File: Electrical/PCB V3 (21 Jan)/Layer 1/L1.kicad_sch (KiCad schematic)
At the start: 218 parts, among them J1 Conn_01x05, Q1 NMOS, U1 LM2587S-ADJ, U2 CD74HC4067SM, U3 CD74HC4067SM, U4 XT30UPB-M, U5 113991054

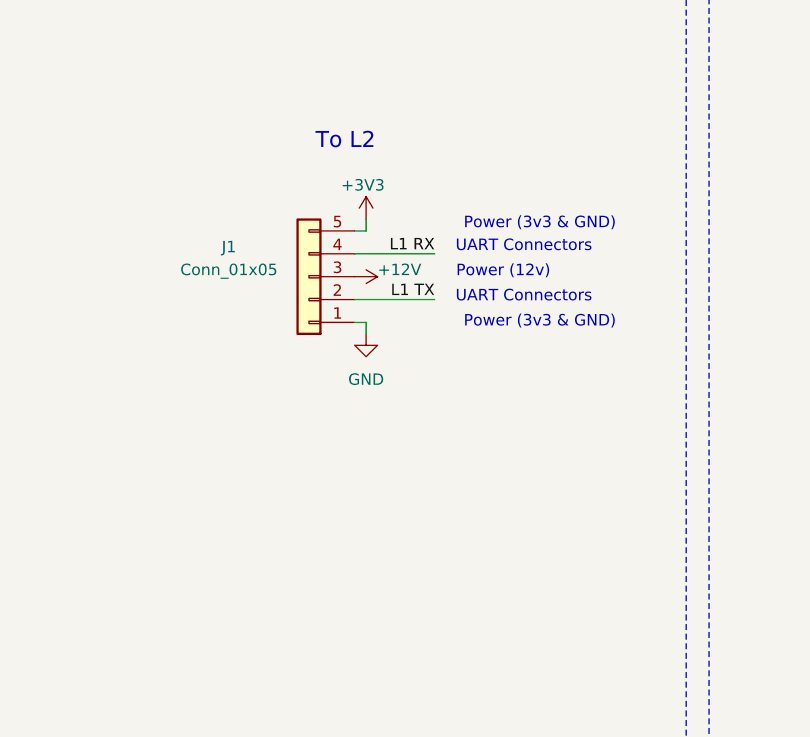
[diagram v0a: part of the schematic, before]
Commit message: 2 new jsts
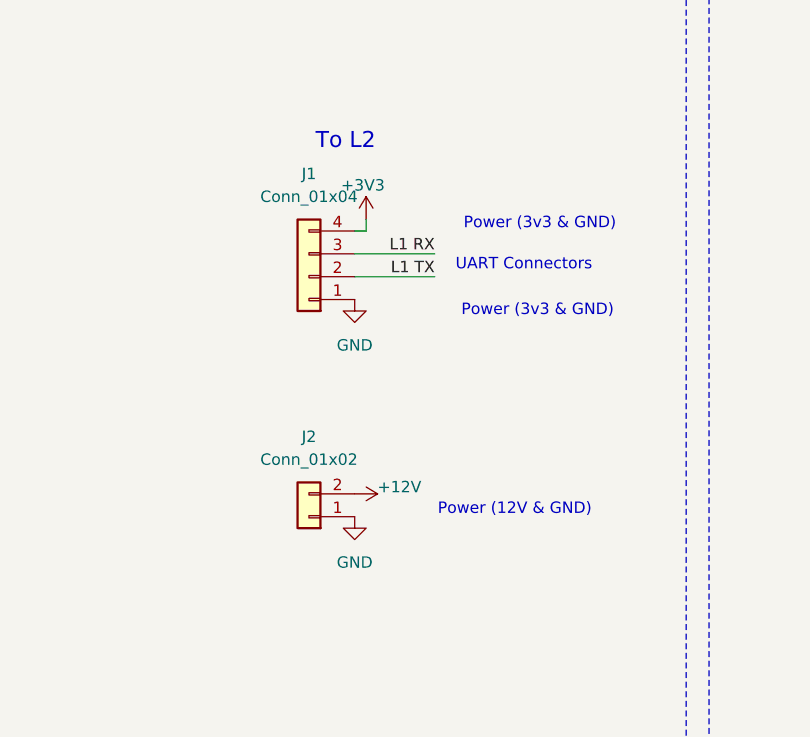
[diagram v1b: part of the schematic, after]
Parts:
- removed J1: Conn_01x05, Connector_JST:JST_EH_B5B-EH-A_1x05_P2.50mm_Vertical, symbol Connector_Generic:Conn_01x05
- added J1: Conn_01x04, Connector_JST:JST_EH_B4B-EH-A_1x04_P2.50mm_Vertical, symbol Connector_Generic:Conn_01x04
- added J2: Conn_01x02, Connector_JST:JST_EH_B2B-EH-A_1x02_P2.50mm_Vertical, symbol Connector_Generic:Conn_01x02
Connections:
- net +12V: now also J2.2 (Pin_2)
- net +3V3: now also J1.4 (Pin_4)
- net GND: now also J1.1 (Pin_1), J2.1 (Pin_1)
- net L1 RX: now also J1.3 (Pin_3)
- net L1 TX: now also J1.2 (Pin_2)
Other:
- note added: "Power (12V & GND)"
- note removed: "Power (12v)"

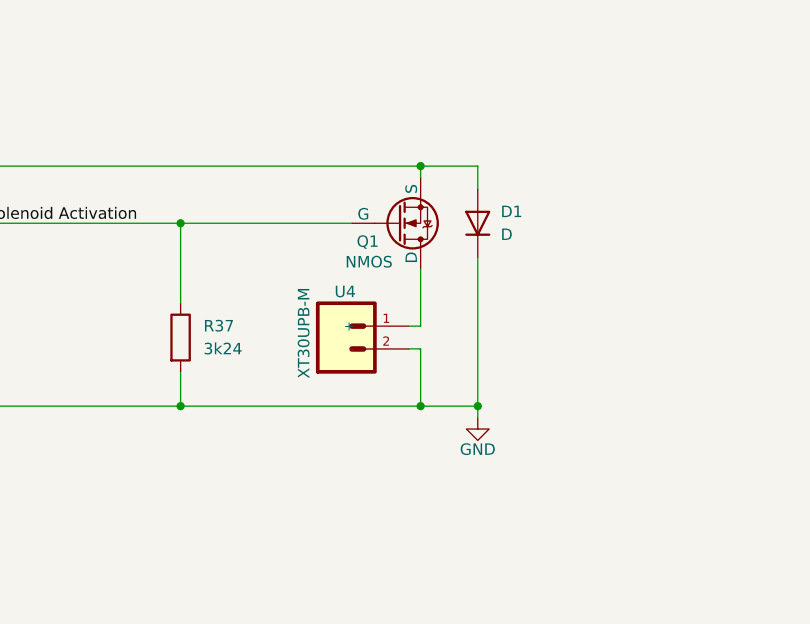
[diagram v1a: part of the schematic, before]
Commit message: redid l1
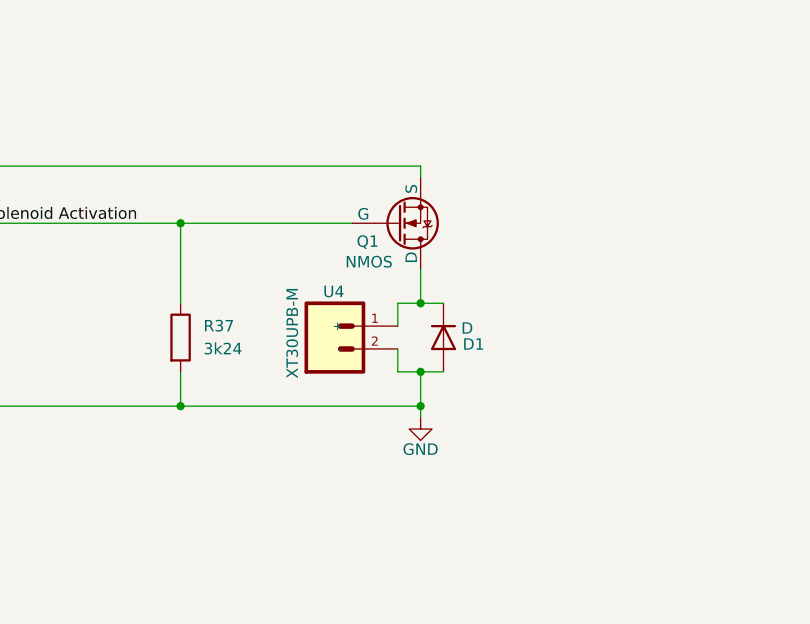
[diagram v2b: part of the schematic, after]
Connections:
- net +24V: no longer D1.2 (A)
- net GND: now also D1.2 (A); no longer D1.1 (K)
- net at Q1.1 (D), U4.1 (+): now also D1.1 (K)
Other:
- moved on the sheet: D1, U4
